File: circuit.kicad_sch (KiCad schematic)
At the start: 73 parts, among them J1 1725656, J2 CTX 3V3 GND TX, J3 CRX 3V3 GND RX, J4 PICO GP4/GP5 CAN, J5 2171750001, Q1 PMV100EPAR, U1 SN65HVD230DR, U2 AMS1117-3.3_C347222

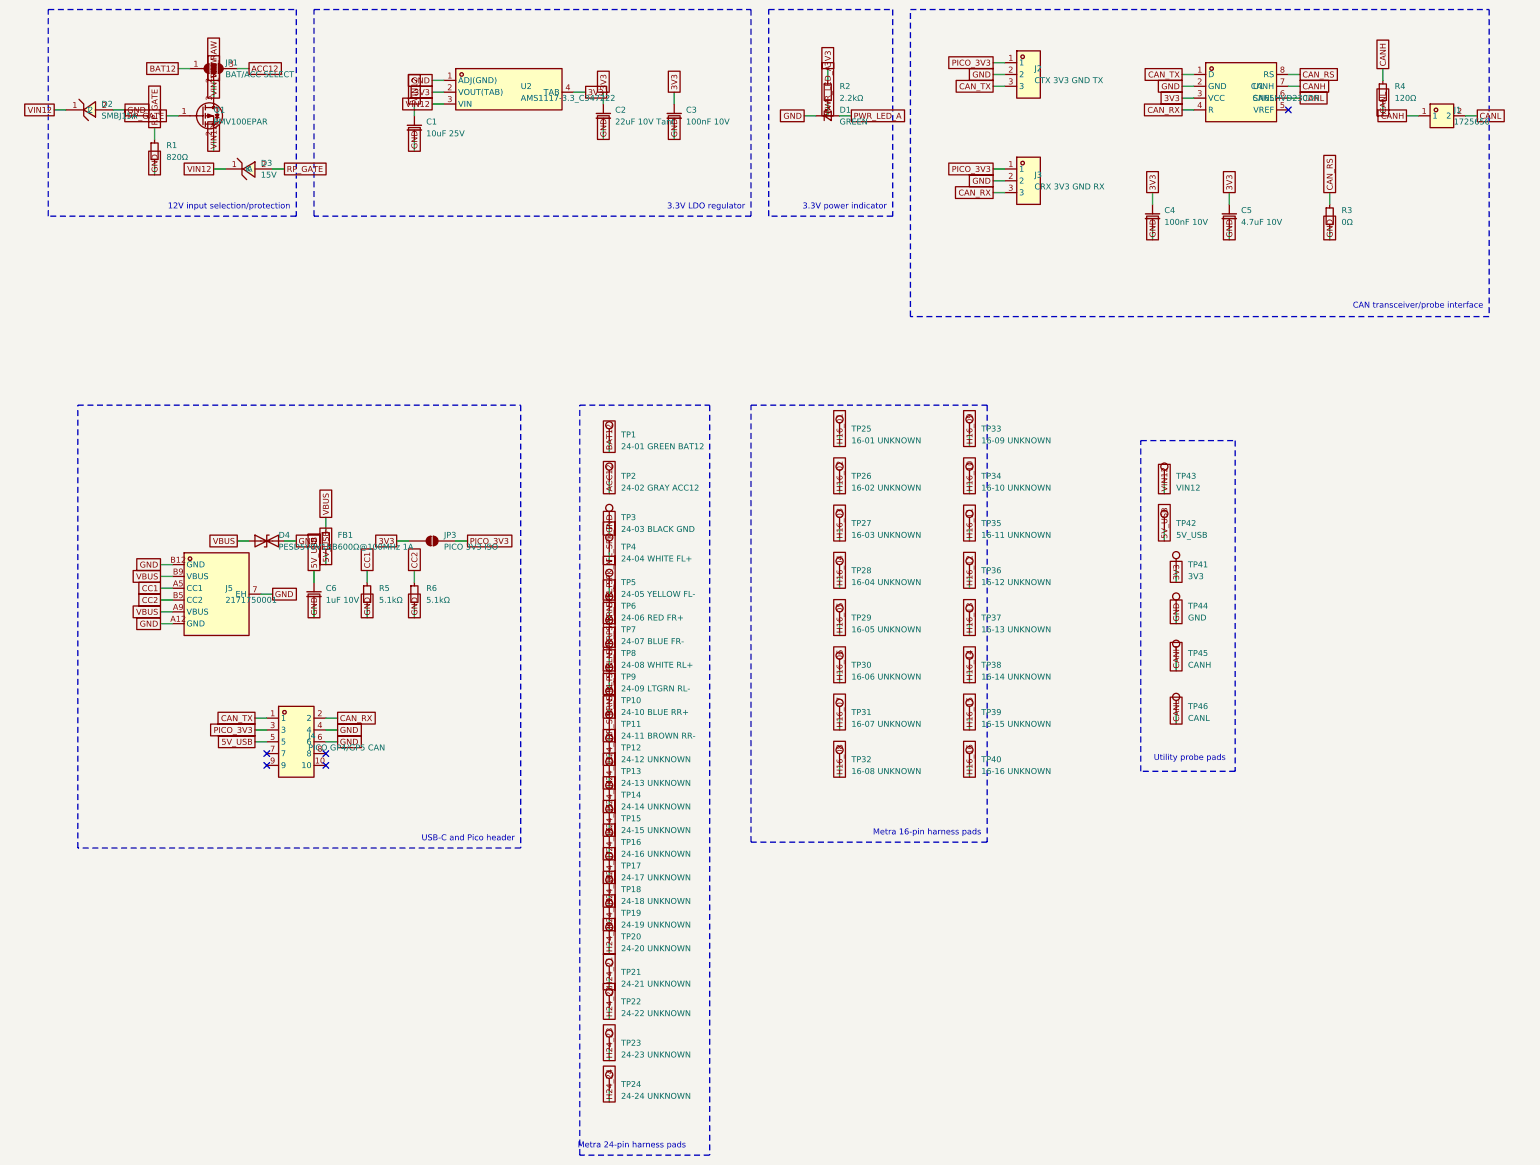
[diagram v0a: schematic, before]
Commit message: more updates
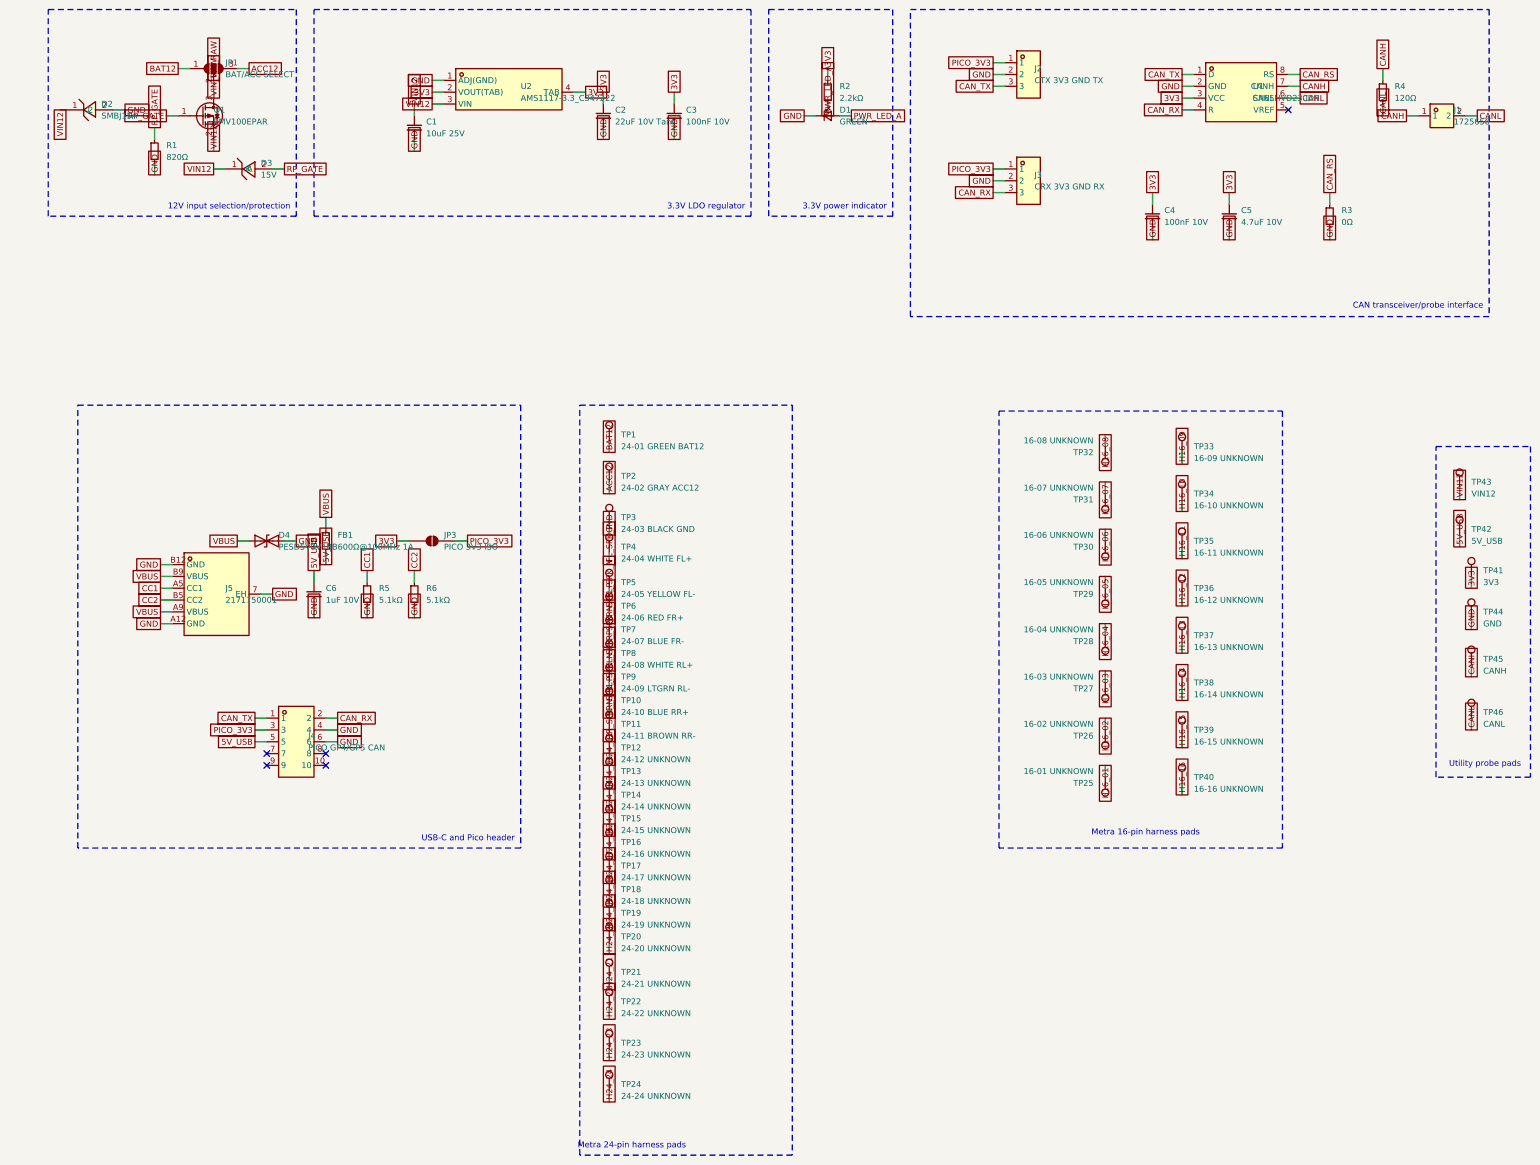
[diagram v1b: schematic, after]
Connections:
- net VIN_RAW: no longer JP1.2 (C), Q1.3 (D)
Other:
- moved on the sheet: TP25, TP26, TP27, TP28, TP29, TP30, TP31, TP32, TP33, TP34, TP35, TP36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

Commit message: pcb finishing
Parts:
- removed J2: CTX 3V3 GND TX, Library:CONN-TH_705430002, symbol Library:705430002
- removed J3: CRX 3V3 GND RX, Library:CONN-TH_705430002, symbol Library:705430002
- R4: now not fitted
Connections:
- net VIN_RAW: now also JP1.2 (C), Q1.3 (D)
- net CC1: no longer names the net of J5.A5 (CC1), R5.1
- net FL_SPK_N: no longer names the net of TP5.1
- net FL_SPK_P: no longer names the net of TP4.1
- net FR_SPK_N: no longer names the net of TP7.1
- net FR_SPK_P: no longer names the net of TP6.1
- net H16_01: no longer names the net of TP25.1
- net H16_02: no longer names the net of TP26.1
- net H16_03: no longer names the net of TP27.1
- net H16_04: no longer names the net of TP28.1
- net H16_05: no longer names the net of TP29.1
- net H16_06: no longer names the net of TP30.1
- net H16_07: no longer names the net of TP31.1
- net H16_08: no longer names the net of TP32.1
- net H16_09: no longer names the net of TP33.1
- net H16_10: no longer names the net of TP34.1
- net H16_11: no longer names the net of TP35.1
- net H16_12: no longer names the net of TP36.1
- net H16_13: no longer names the net of TP37.1
- net H16_14: no longer names the net of TP38.1
- net H16_15: no longer names the net of TP39.1
- net H16_16: no longer names the net of TP40.1
- net H24_12: no longer names the net of TP12.1
- net H24_13: no longer names the net of TP13.1
- net H24_14: no longer names the net of TP14.1
- net H24_15: no longer names the net of TP15.1
- net H24_16: no longer names the net of TP16.1
- net H24_17: no longer names the net of TP17.1
- net H24_18: no longer names the net of TP18.1
- net H24_19: no longer names the net of TP19.1
- net H24_20: no longer names the net of TP20.1
- net H24_21: no longer names the net of TP21.1
- net H24_22: no longer names the net of TP22.1
- net H24_23: no longer names the net of TP23.1
- net H24_24: no longer names the net of TP24.1
- net RL_SPK_N: no longer names the net of TP9.1
- net RL_SPK_P: no longer names the net of TP8.1
- net RP_GATE: no longer names the net of D3.2 (A), Q1.1 (G), R1.1
- net RR_SPK_N: no longer names the net of TP11.1
- net RR_SPK_P: no longer names the net of TP10.1
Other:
- note added: "12V input protection"
- note added: "3.3V regulator"
- note added: "3V3 power indicator"
- note added: "CAN transceiver interface"
- note added: "Metra 16-pin pads"
- note added: "Metra 24-pin pads"
- note added: "Pico USB/header power"
- note removed: "12V input selection/protection"
- note removed: "3.3V LDO regulator"
- note removed: "3.3V power indicator"
- note removed: "CAN transceiver/probe interface"
- note removed: "Metra 16-pin harness pads"
- note removed: "Metra 24-pin harness pads"
- note removed: "USB-C and Pico header"
- company: Jasper Mayone -> (none)
- title: Mazzy Harness Probe -> (none)
